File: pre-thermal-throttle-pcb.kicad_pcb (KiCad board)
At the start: 2 copper layers, 113.4 x 100.3 mm, 70 parts, among them IC1 LMR51420XFDDCR, IC2 ADR02BRZ-REEL7, IC3 ADR02BRZ-REEL7, IC4 ADR02BRZ-REEL7, IC5 ADR02BRZ-REEL7, J1 RJHSE-5381-ND, J2 STEERING, J3 Motor Throttle Connector, J4 RJHSE-5381-ND, U1 SN65HVD230, U2 BMI088, U3 MAX3485CSA, U4 MCP3008, U5 ESP32-DevKitC

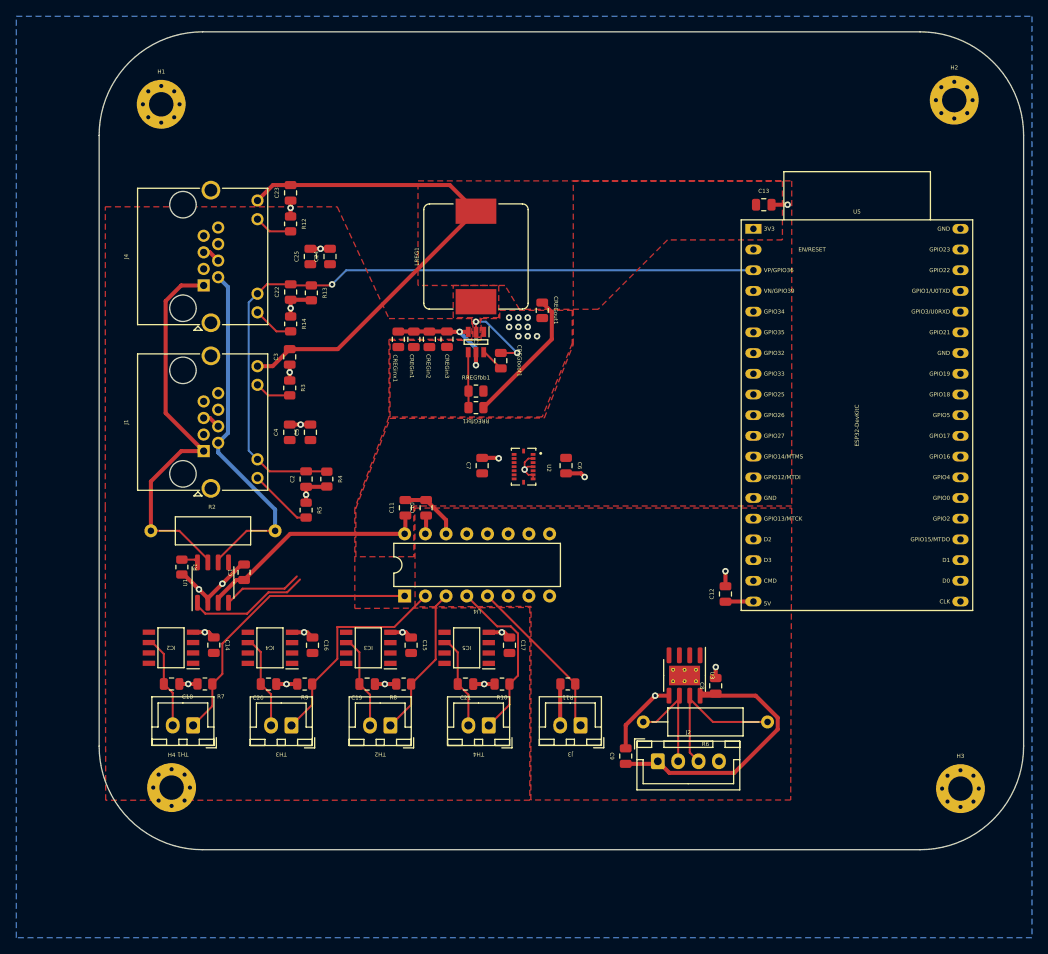
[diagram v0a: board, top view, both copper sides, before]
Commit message: Hopefully finished?
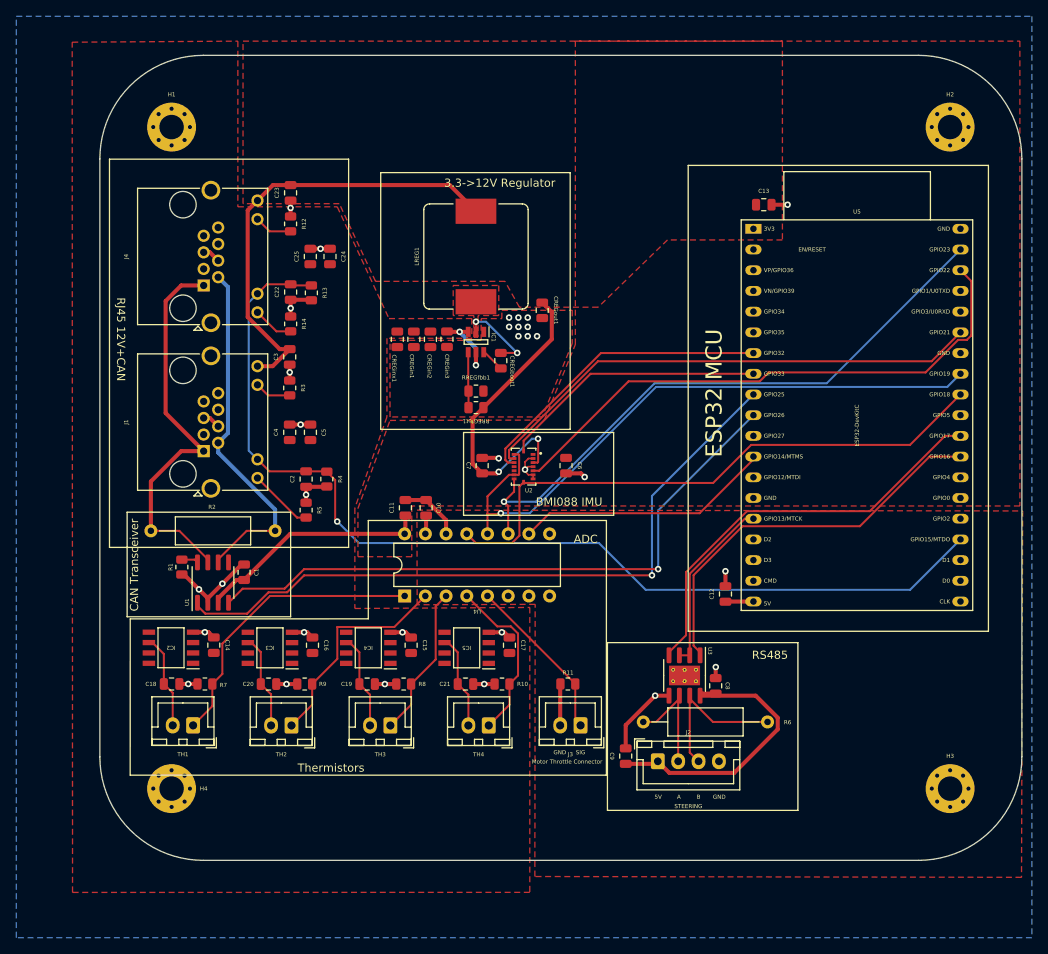
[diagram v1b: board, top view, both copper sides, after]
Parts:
- moved H2 3.34 mm to (237.7, 49.1)
- moved H1 3.07 mm to (142.2, 49.1)
- moved H3 1.27 mm to (237.7, 130.3)
- moved CREGin2 0.13 mm to (174.0, 75.2)
- moved CREGinx1 0.13 mm to (169.9, 75.2)
- moved H4 0.13 mm to (142.2, 130.3)
- renumbered IC4 to IC3, IC3 to IC4, TH3 to TH2, TH2 to TH3
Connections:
- U5 pad 12: unconnected-(U5-Pad12) -> ESP ADC CS
- U5 pad 15: unconnected-(U5-Pad15) -> RS485 RTS
- U5 pad 21: IMU_INT1 -> unconnected-(U5-Pad21)
- U5 pad 22: IMU_INT2 -> unconnected-(U5-Pad22)
- U5 pad 23: unconnected-(U5-Pad23) -> ESP_OK_LED
- U5 pad 3: ESP_OK_LED -> unconnected-(U5-Pad3)
- U5 pad 4: ESP ADC CS -> unconnected-(U5-Pad4)
- U5 pad 5: RS485 RTS -> unconnected-(U5-Pad5)
- U5 pad 7: unconnected-(U5-Pad7) -> IMU_INT2
- U5 pad 8: unconnected-(U5-Pad8) -> IMU_INT1
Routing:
- net ESP CIPO: track 0.00 -> 77.8 mm, vias 0 -> 1
- net ESP COPI: track 0.00 -> 76.3 mm, vias 0 -> 1
- net ESP SPI CLK: track 0.00 -> 72.2 mm
- net CAN_TXD: track 15.1 -> 85.8 mm, vias 0 -> 1
- net ESP Gyro CS: track 0.00 -> 69.2 mm
- net CAN_RXD: track 9.72 -> 78.1 mm, vias 0 -> 1
- net ESP Accel : track 0.00 -> 63.0 mm
- net TXD2: track 0.00 -> 51.7 mm
- net RXD2: track 0.00 -> 48.9 mm
- net IMU_INT2: track 0.00 -> 37.9 mm
- net ESP_OK_LED: track 92.5 -> 126.6 mm
- net IMU_INT1: track 0.00 -> 32.9 mm
- net ESP ADC CS: track 0.00 -> 31.7 mm
- net RS485 RTS: track 0.00 -> 21.9 mm
- net +3.3V: track 109.4 -> 122.4 mm, vias 0 -> 2
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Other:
- board size 113.4 x 100.3 mm -> 113.1 x 98.8 mm
- board text added: "3.3->12V Regulator"
- board text added: "5V"
- board text added: "A"
- board text added: "ADC"
- board text added: "B"
- board text added: "BMI088 IMU"
- board text added: "CAN Transceiver"
- board text added: "ESP32 MCU"
- board text added: "GND"
- board text added: "RJ45 12V+CAN"
- board text added: "RS485"
- board text added: "SIG"
- board text added: "Thermistors"
